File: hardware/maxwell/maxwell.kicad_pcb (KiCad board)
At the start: 2 copper layers, 124 x 60 mm, 81 parts, among them J1 Canbus 1, J10 SPI2_B, J11 BACKUP, J12 UART4, J13 UART5, J14 I2C1, J15 GPIO, J16 ESP_BM, J17 ESP_PROG, J18 Supercap, J2 Canbus 2, J3 Neopixel, J4 BOOT0, J5 SPI2_A, J6 Programmer, J7 Dynamo Input, J8 BOOT1, J9 Battery, Q1 BSS138, Q2 PSMN5R4-25YLD, Q3 NTR1P02T1, Q4 NTR1P02T1, Q5 NTR1P02T1, U1 MCP1501, U10 MIC39102, U2 SN65HVD233, U3 TPS2113, U5 ESP-32S, U7 STM32F103RETx, U8 TLP188, U9 Buck Regulator, Y1 32.768k, Y2 8M

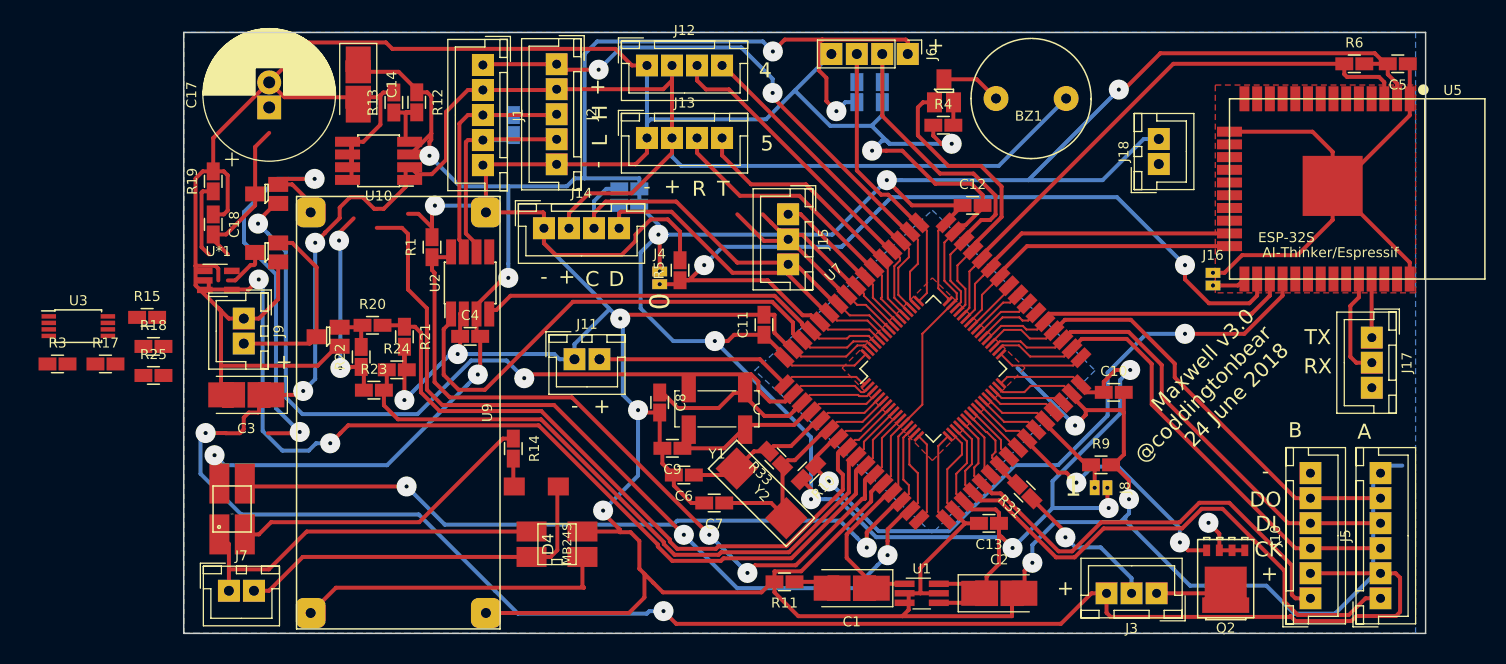
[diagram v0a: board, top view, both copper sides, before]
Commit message: v1.5 ready for production.
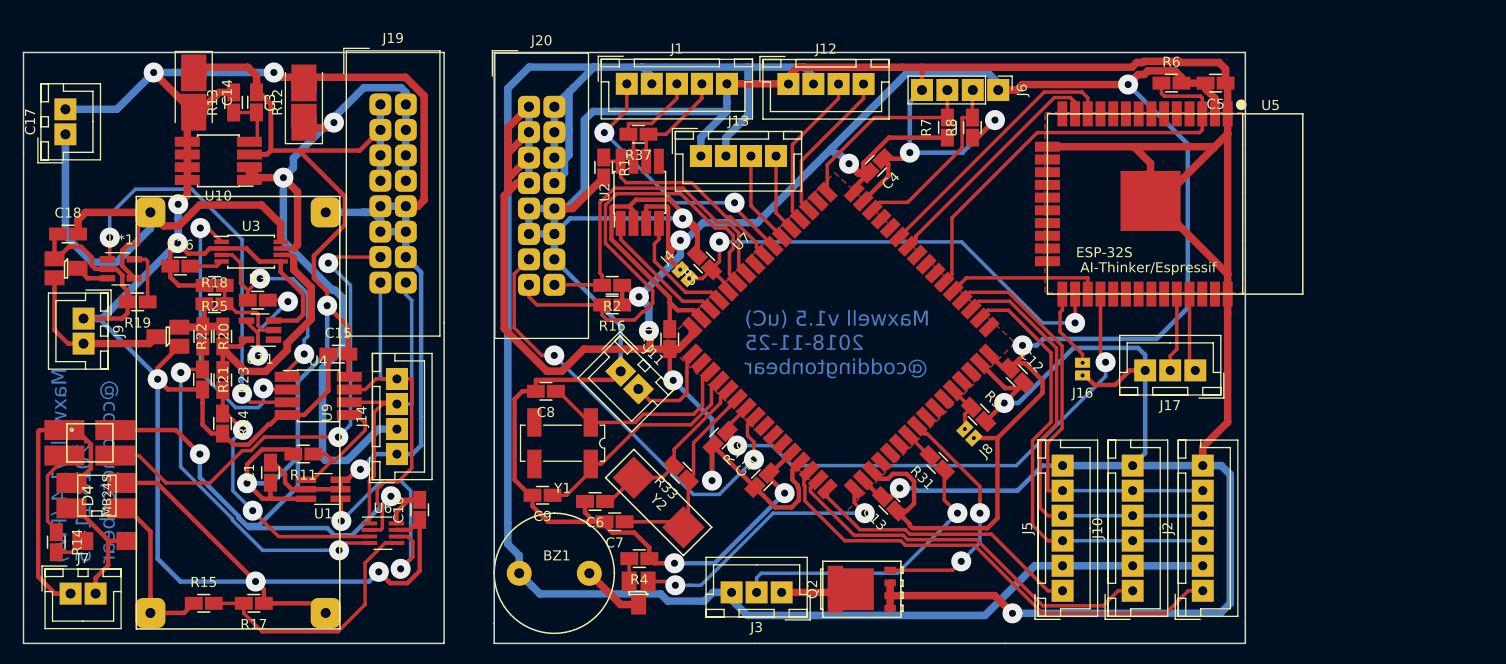
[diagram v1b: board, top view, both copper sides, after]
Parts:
- removed C2: 2.2u, coddingtonbear:CP_Tantalum_Case-C_EIA-6032-28_Milling
- removed J15: GPIO, coddingtonbear:JST_XH_B03B-XH-A_03x2.50mm_Straight_LargePads
- removed J18: Supercap, coddingtonbear:JST_XH_B02B-XH-A_02x2.50mm_Straight_LargePads
- removed Q3: NTR1P02T1, coddingtonbear:SOT-23_LargePads
- added C15: 0.1u, coddingtonbear:0805_Milling, F.Cu at (88.4, 103.1)
- added C16: 0.1u, coddingtonbear:0805_Milling, F.Cu at (96.6, 118.7)
- added J19: Interconnect (Power), coddingtonbear:IDC-Header_2x08_P2.54mm_Vertical_Largepads, F.Cu at (92.6, 78.2)
- added J20: Interconnect (uC), coddingtonbear:IDC-Header_2x08_P2.54mm_Vertical_Largepads, F.Cu at (107.5, 78.4)
- added R26: 250, coddingtonbear:0805_Milling, F.Cu at (72.7, 94.3)
- added U11: SN74LVC1G14DBVR, Package_TO_SOT_SMD:SOT-23-5_HandSoldering, F.Cu at (80.6, 100.7)
- added U4: PCA9536D, coddingtonbear:SOIC-8_3.9x4.9mm_P1.27mm_LargePads, F.Cu at (86.4, 107.3)
- added U6: AD7995, Package_TO_SOT_SMD:SOT-23-8_Handsoldering, F.Cu at (92.9, 121.0)
- C1: value 2.2u -> 0.1u; footprint coddingtonbear:CP_Tantalum_Case-C_EIA-6032-28_Milling -> coddingtonbear:0805_Milling
- C17: footprint Capacitor_THT:CP_Radial_D13.0mm_P2.50mm -> coddingtonbear:JST_XH_B02B-XH-A_02x2.50mm_Straight_LargePads
- J2: value Canbus 2 -> SPI2_C; footprint coddingtonbear:JST_XH_B05B-XH-A_05x2.50mm_Straight_LargePads -> coddingtonbear:JST_XH_B06B-XH-A_06x2.50mm_Straight_LargePads
- R11: value 50 -> 10k
- R16, R2, R37, R7, R8: moved to F.Cu
- R18: value ANY -> 2k
- R25: value ANY -> 1k
- R3: value 500 -> 10k
- U7: footprint kicad-castellated-breakouts:QFP64-1.27MM-CASTELLATED-VERS -> kicad-castellated-breakouts:QFP64-1.27MM-CASTELLATED
- moved J2 83.2 mm to (174.8, 126.8), turned to 90 degrees
- moved BZ1 67.2 mm to (110.0, 125.0), turned to 0 degrees
- moved U1 60.6 mm to (86.9, 116.6), turned to 180 degrees
- moved C1 59.2 mm to (81.7, 115.0), turned to 90 degrees
- moved Q1 58.7 mm to (118.4, 127.0), turned to 270 degrees
- moved R4 52.9 mm to (118.5, 123.5), turned to 180 degrees
- moved R11 49.7 mm to (84.9, 113.1)
- moved R14 46.6 mm to (60.3, 121.9)
- moved D4 46.2 mm to (64.3, 117.2)
- moved C4 43.9 mm to (142.1, 84.3), turned to 225 degrees
- moved D1 43.4 mm to (65.1, 121.8)
- moved J3 37.4 mm to (132.7, 126.9)
- moved Q2 36.3 mm to (140.7, 126.6), turned to 90 degrees
- moved C10 36.2 mm to (130.7, 115.7), turned to 45 degrees
- moved J5 31.8 mm to (160.8, 126.8)
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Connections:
- net Net-(J9-Pad2) renamed /Power/BATT_PRE_POLARITY
- net Net-(Q4-Pad3) renamed /Power/BATT_CHARGE_PRE_POLARITY
- C1 pad 1: Net-(C1-Pad1) -> +3V3
- C1 pad 2: Net-(C1-Pad2) -> GND
- C17 pad 1: /Power/Batt_Charge -> /Power/+Dynamo_Buck
- C18 pad 2: /Power/Batt_Charge -> /Power/+Dynamo_Buck
- J2 pad 1: POWER_ON -> SPI2_CS_C
- J2 pad 3: /CAN+ -> SPI2_SCK
- J2 pad 4: /CAN- -> SPI2_MISO
- J2 pad 5: GND -> SPI2_MOSI
- Q5 pad 2: Net-(Q5-Pad2) -> /Power/BATT_PRE_SENSE
- R11 pad 1: Net-(C1-Pad2) -> ENABLE_VREF
- R11 pad 2: GND -> +3V3
- R18 pad 1: /Power/+Dynamo_Buck -> /Power/BATT_PRE_SENSE
- R18 pad 2: DYNAMO_BUCK_VOLTAGE -> ~BATT_DISABLE
- R20 pad 1: Net-(Q5-Pad2) -> /Power/BATT_PRE_SENSE
- R22 pad 2: Net-(Q5-Pad2) -> /Power/BATT_PRE_SENSE
- R25 pad 1: GND -> ~BATT_DISABLE
- R25 pad 2: DYNAMO_BUCK_VOLTAGE -> GND
- R3 pad 1: GND -> BATTERY_SOURCE_DISABLE
- U*1 pad 4: /Power/Batt_Charge -> /Power/+Dynamo_Buck
- U1 pad 1: Net-(C1-Pad1) -> Net-(U1-Pad1)
- U1 pad 4: +3V3 -> ENABLE_VREF
- U2 pad 5: Net-(U2-Pad5) -> (no net)
- U3 pad 1: Net-(U3-Pad1) -> POWER_SOURCE_INDICATOR
- U3 pad 3: DYNAMO_SOURCE_DISABLE -> BATTERY_SOURCE_DISABLE
- U3 pad 4: Net-(R3-Pad2) -> Net-(R26-Pad2)
- U3 pad 6: /Power/+Dynamo_Buck -> +BATT
- U3 pad 8: +BATT -> /Power/+Dynamo_Buck
- U5 pad 10: Net-(U5-Pad10) -> (no net)
- U5 pad 11: Net-(U5-Pad11) -> (no net)
- U5 pad 12: Net-(U5-Pad12) -> BT_DO
- U5 pad 13: Net-(U5-Pad13) -> BT_DI
- U5 pad 14: Net-(U5-Pad14) -> (no net)
- U5 pad 16: Net-(U5-Pad16) -> (no net)
- U5 pad 17: Net-(U5-Pad17) -> (no net)
- U5 pad 18: Net-(U5-Pad18) -> (no net)
- U5 pad 19: Net-(U5-Pad19) -> (no net)
- U5 pad 20: Net-(U5-Pad20) -> (no net)
- U5 pad 21: Net-(U5-Pad21) -> (no net)
- U5 pad 22: Net-(U5-Pad22) -> (no net)
- U5 pad 23: BT_DO -> (no net)
- U5 pad 24: BT_DI -> (no net)
- U5 pad 29: Net-(U5-Pad29) -> (no net)
- U5 pad 30: Net-(U5-Pad30) -> (no net)
- U5 pad 31: Net-(U5-Pad31) -> (no net)
- U5 pad 32: Net-(U5-Pad32) -> (no net)
- U5 pad 33: Net-(U5-Pad33) -> (no net)
- U5 pad 36: Net-(U5-Pad36) -> (no net)
- U5 pad 37: Net-(U5-Pad37) -> (no net)
- U5 pad 4: Net-(U5-Pad4) -> (no net)
- U5 pad 5: Net-(U5-Pad5) -> (no net)
- U5 pad 6: Net-(U5-Pad6) -> (no net)
- U5 pad 7: Net-(U5-Pad7) -> (no net)
- U5 pad 8: Net-(U5-Pad8) -> (no net)
- U5 pad 9: Net-(U5-Pad9) -> (no net)
- U7 pad 10: ~BATT_CHARGING -> (no net)
- U7 pad 11: CAN_DISABLE -> (no net)
- U7 pad 13: Net-(C1-Pad1) -> +3V3
- U7 pad 14: SPEED -> SPI2_CS_C
- U7 pad 15: DYNAMO_SOURCE_DISABLE -> SPI2_CS_B
- U7 pad 17: SPI2_CS_B -> BUZZER
- U7 pad 2: ~BATT_CHARGE_ENABLE -> (no net)
- U7 pad 20: Net-(U7-Pad20) -> (no net)
- U7 pad 21: Net-(U7-Pad21) -> (no net)
- U7 pad 22: Net-(U7-Pad22) -> (no net)
- U7 pad 24: DYNAMO_VOLTAGE -> ENABLE_BATT_POWER
- U7 pad 25: DYNAMO_BUCK_VOLTAGE -> (no net)
- U7 pad 26: ENABLE_BATT_POWER -> (no net)
- U7 pad 27: Net-(U7-Pad27) -> (no net)
- U7 pad 29: GPS_DI -> (no net)
- U7 pad 30: GPS_DO -> (no net)
- U7 pad 33: Net-(U7-Pad33) -> (no net)
- U7 pad 38: Net-(U7-Pad38) -> ~DISABLE_ESP
- U7 pad 39: Net-(U7-Pad39) -> (no net)
- U7 pad 40: Net-(U7-Pad40) -> (no net)
- U7 pad 41: Net-(U7-Pad41) -> (no net)
- U7 pad 44: ~DISABLE_ESP -> (no net)
- U7 pad 45: BUZZER -> (no net)
- U7 pad 50: POWER_ON -> (no net)
- U7 pad 55: Net-(J15-Pad1) -> POWER_ON
- U7 pad 56: Net-(J15-Pad2) -> CAN_DISABLE
- U7 pad 57: Net-(J15-Pad3) -> (no net)
- U7 pad 8: BATT_VOLTAGE -> SPEED
- U7 pad 9: CURRENT_SENSE -> (no net)
- Y1 pad 2: Net-(Y1-Pad2) -> (no net)
- Y1 pad 3: Net-(Y1-Pad3) -> (no net)
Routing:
- net GND: track 698.3 -> 808.6 mm, vias 12 -> 16
- net DYNAMO_SOURCE_DISABLE: track 89.6 -> 0.00 mm, vias 2 -> 0
- net ~BATT_CHARGE_ENABLE: track 86.4 -> 0.00 mm, vias 2 -> 0
- net ~BATT_CHARGING: track 100.9 -> 41.1 mm
- net CAN_DISABLE: track 78.6 -> 21.3 mm, vias 2 -> 0
- net I2C1_SDA: track 35.4 -> 84.2 mm
- net SPI2_CS_C: track 0.00 -> 48.6 mm
- net CAN_TX: track 56.8 -> 13.4 mm
- net BOOT0: track 92.8 -> 50.3 mm
- net SPI2_CS_A: track 69.2 -> 28.2 mm
- net CURRENT_SENSE: track 69.1 -> 29.2 mm, vias 0 -> 2
- net BATT_VOLTAGE: track 72.2 -> 36.7 mm, vias 0 -> 2
- net POWER_ON: track 60.6 -> 27.6 mm
- net CAN_RX: track 41.5 -> 12.0 mm
- net POWER_SOURCE_INDICATOR: track 0.00 -> 28.9 mm, vias 0 -> 2
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- removed copper zone on B.Cu, net GND
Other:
- board size 124 x 60 mm -> 122 x 59 mm
- net class Default: trace_width 0.4 -> 0.35; via_drill 0.4 -> 0.7
- net class Power added: clearance 0.2, trace_width 0.45, via_dia 2, via_drill 0.7
- board text added: "Maxwell v1.4 (Pwr) 2018-11-25 @coddingtonbear"
- board text added: "Maxwell v1.5 (uC) 2018-11-25 @coddingtonbear"
- board text removed: "+"
- board text removed: "-"
- board text removed: "0"
- board text removed: "1"
- board text removed: "4"
- board text removed: "5"
- board text removed: "A"
- board text removed: "B"
- board text removed: "C"
- board text removed: "CK"
- board text removed: "D"
- board text removed: "DI"
- board text removed: "DO"
- board text removed: "H"
- board text removed: "L"
- board text removed: "Maxwell v3.0 @coddingtonbear 24 June 2018"
- board text removed: "R"
- board text removed: "RX"
- board text removed: "T"
- board text removed: "TX"
- board text removed: "~"
